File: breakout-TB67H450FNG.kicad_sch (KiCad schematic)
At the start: 8 parts, among them IC1 TB67H450FNG,EL, J1 Conn_01x06, J2 Screw_Terminal_01x02

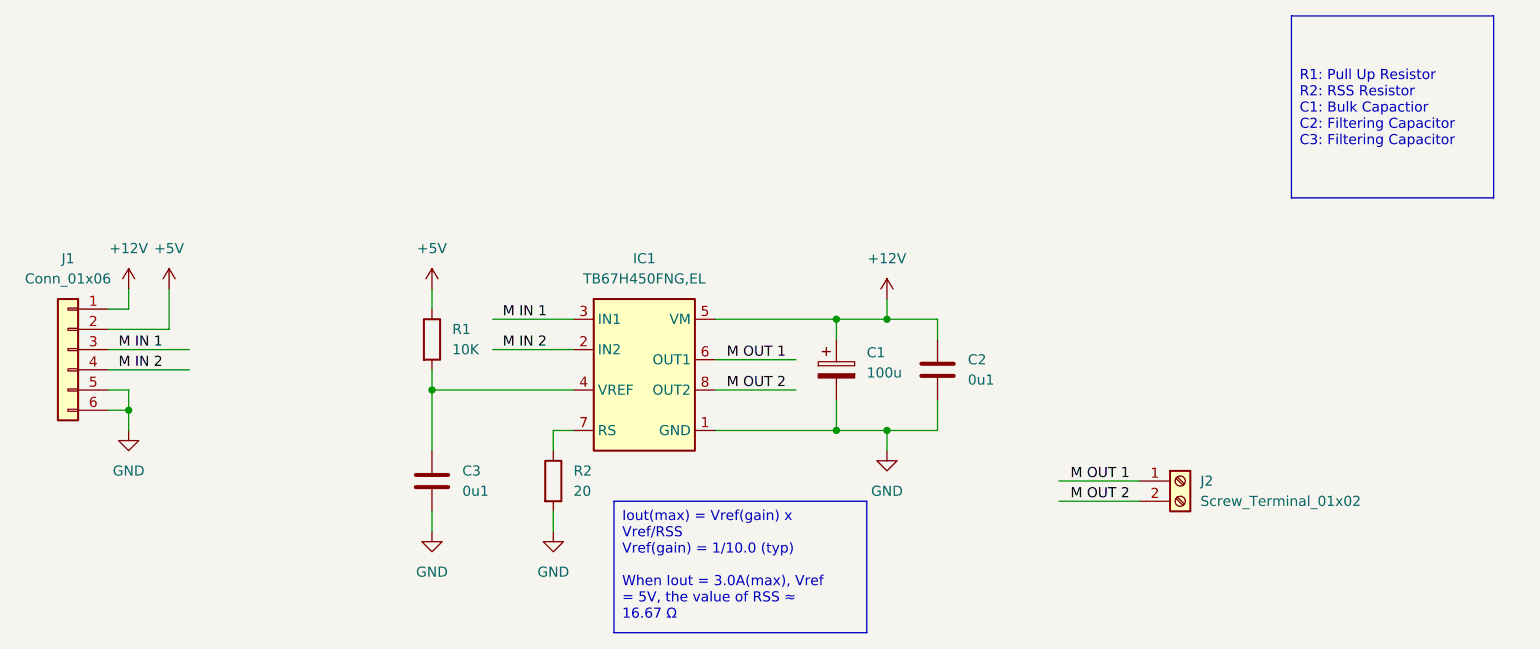
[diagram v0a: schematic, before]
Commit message: uploaded image to readme
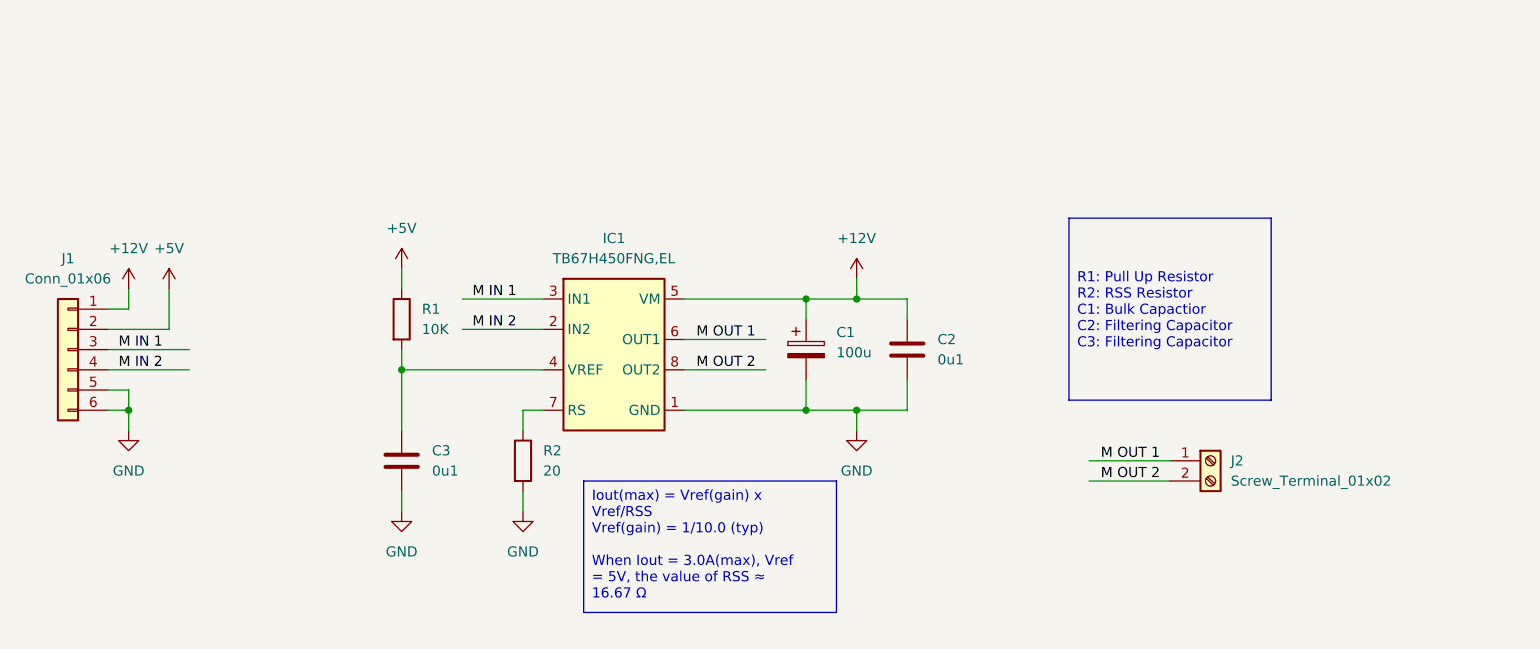
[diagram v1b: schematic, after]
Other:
- company: (none) -> Created by: Vincent Cayadi
- title: (none) -> Breakout TB67H450FNG
- moved on the sheet: C1, C2, C3, IC1, J2, R1, R2
